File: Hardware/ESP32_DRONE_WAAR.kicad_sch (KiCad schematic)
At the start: 62 parts, among them J1 USB_B_Micro, J2 Conn_01x04_MountingPin, J3 Conn_01x04_MountingPin, Q1 S8050, Q2 S8050, SW1 SW_MEC_5G, SW2 SW_MEC_5G, SW3 SW_MEC_5G, U1 CP2104, U2 ESP32-S2-WROVER, U3 LD1117V33, U4 ME6217C33M5G, U5 MPU-9250, U6 LT1962-3.3V LDO

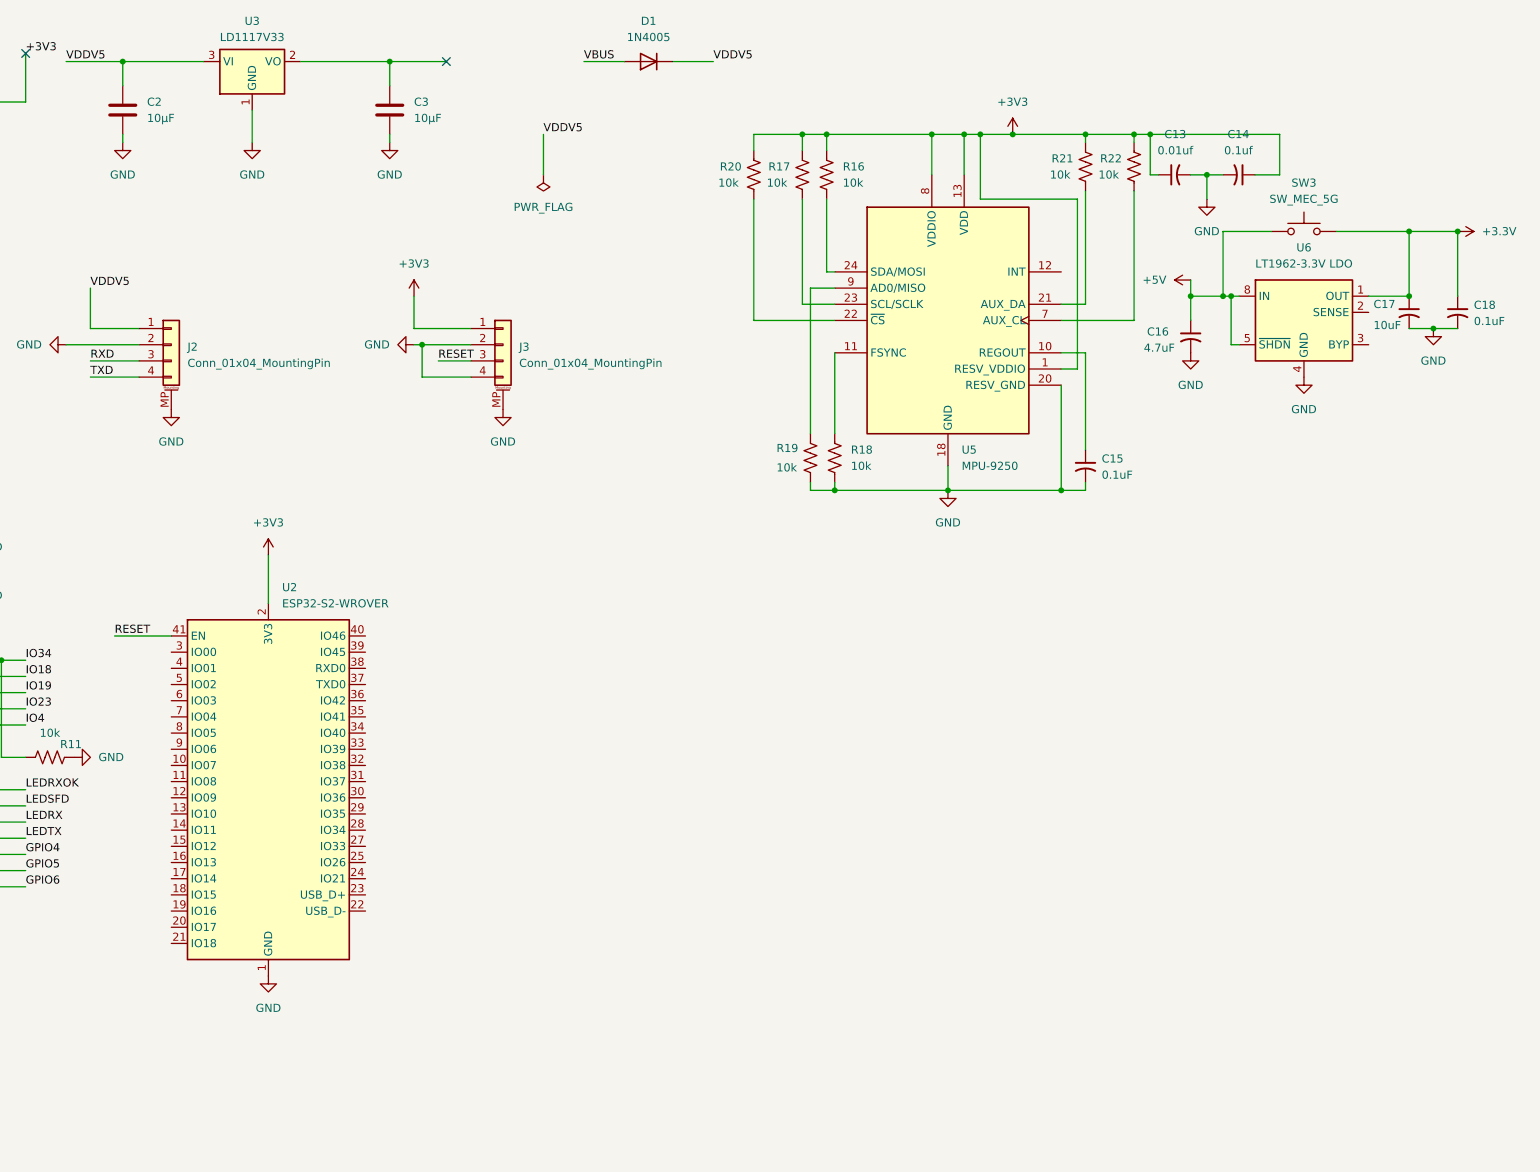
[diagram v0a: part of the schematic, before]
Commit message: Add files via upload
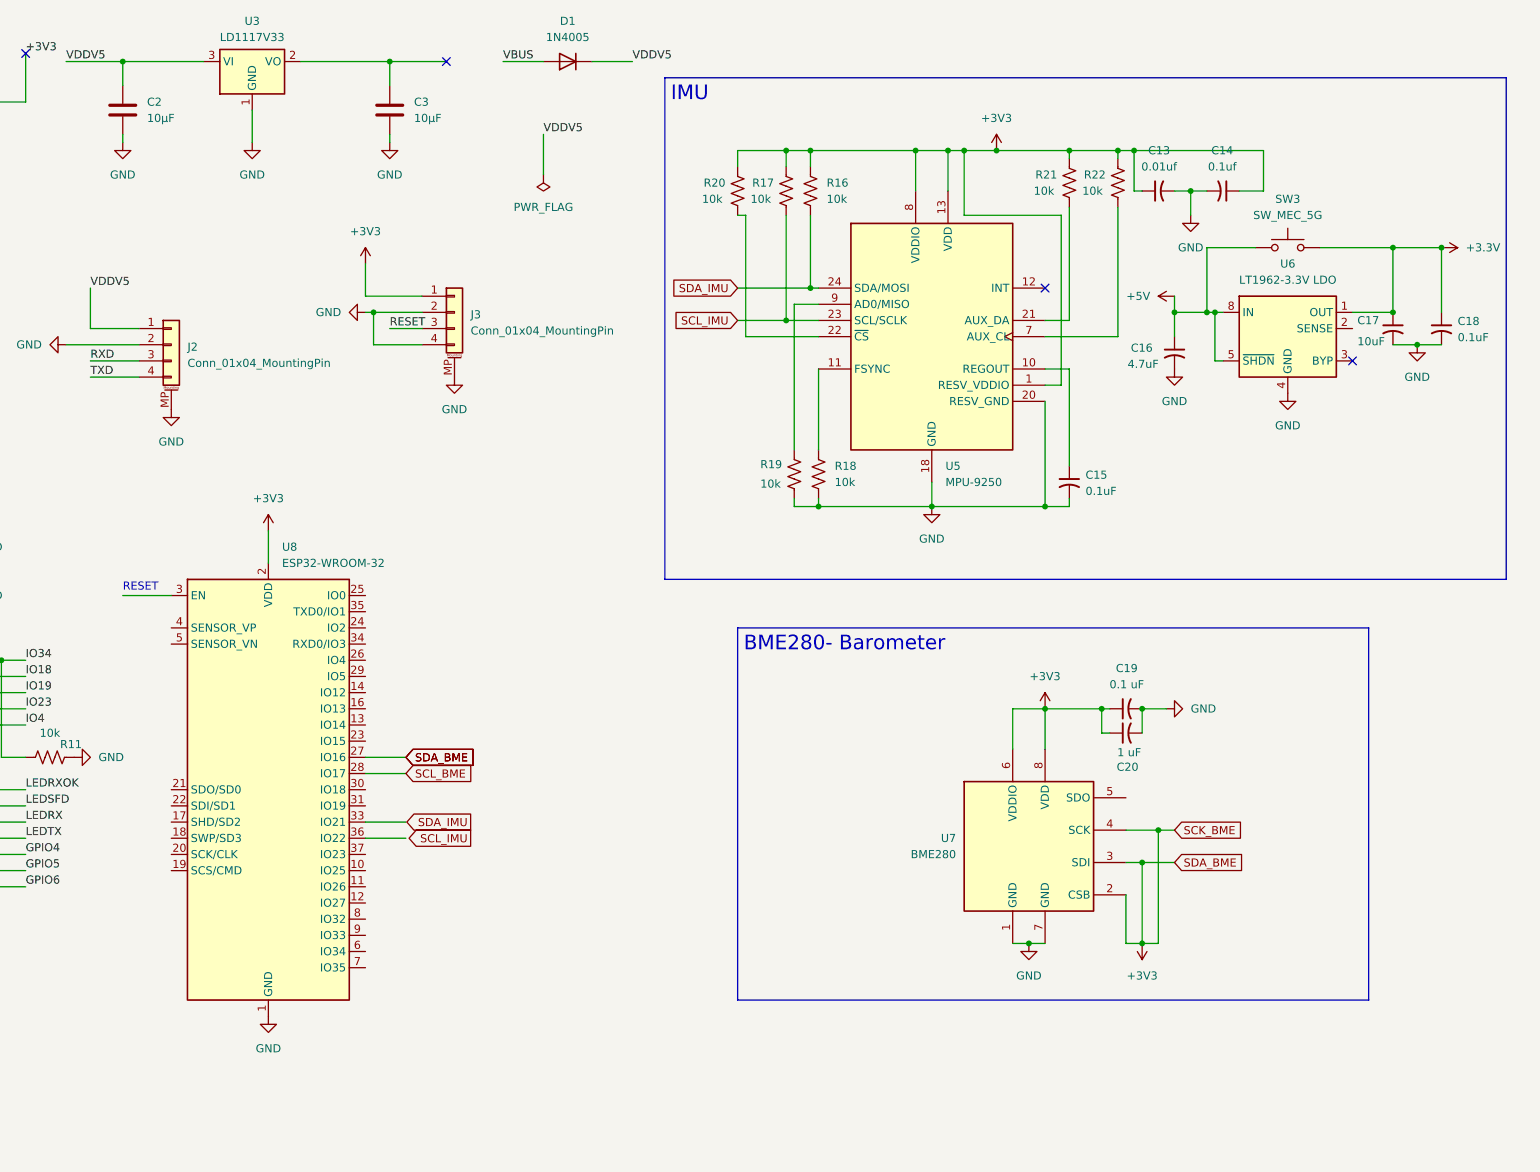
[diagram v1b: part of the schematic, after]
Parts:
- removed U2: ESP32-S2-WROVER, RF_Module:ESP32-S2-WROVER, symbol RF_Module:ESP32-S2-WROVER
- added C19: 0.1 uF, symbol Device:C_Small_US
- added C20: 1 uF, symbol Device:C_Small_US
- added U7: BME280, Sensors:PSON65P250X250X100-8N, symbol Sensor:BME280
- added U8: ESP32-WROOM-32, RF_Module:ESP32-WROOM-32, symbol RF_Module:ESP32-WROOM-32
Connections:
- net +3V3: now also C19.1, C20.1, U7.2 (CSB), U7.3 (SDI), U7.4 (SCK), U7.6 (VDDIO), U7.8 (VDD), U8.2 (VDD), U8.27 (IO16)
- net GND: now also C19.2, C20.2, U7.1 (GND), U7.7 (GND), U8.1 (GND), U8.15 (GND), U8.38 (GND), U8.39 (GND)
- net SDA_IMU: now reaches R16.2, U5.24 (SDA/MOSI)
- net SCL_IMU: now reaches R17.1, U5.23 (SCL/SCLK)
- new net SCL_BME: U8.28 (IO17)
- no-connect marks 15 -> 17
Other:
- note added: "RESET"
- moved on the sheet: C13, C14, C15, C16, C17, C18, D1, J3, R16, R17, R18, R19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
